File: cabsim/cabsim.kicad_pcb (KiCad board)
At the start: 2 copper layers, 87 x 30 mm, 45 parts, among them J1 NJ3FD-V, J3 Conn_01x01, J4 Conn_01x01, J5 NJ3FD-V, U3 Op_Amp_Dual, U4 Opamp_Quad

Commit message: update pcb
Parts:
- C4: value 1n -> 3.3n
- C7: value 2.2n -> 3.3n
- R19: value 390 -> 330
- R5, R9: value 3.9k -> 3.3k
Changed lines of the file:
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@@
 			)
 		)
-		(property "Value" "390"
+		(property "Value" "330"
 			(at 3.81 2.31 90)
 			(layer "F.Fab")
@@
 			)
 		)
-		(property "Value" "3.9k"
+		(property "Value" "3.3k"
 			(at 3.81 2.31 90)
 			(layer "F.Fab")
@@
 			)
 		)
-		(property "Value" "3.9k"
+		(property "Value" "3.3k"
 			(at 3.81 2.31 90)
 			(layer "F.Fab")
@@
 			)
 		)
-		(property "Value" "2.2n"
+		(property "Value" "3.3n"
 			(at 2.5 -2.31 90)
 			(layer "B.Fab")
@@
 			)
 		)
-		(property "Value" "1n"
+		(property "Value" "3.3n"
 			(at 2.5 -2.31 90)
 			(layer "B.Fab")

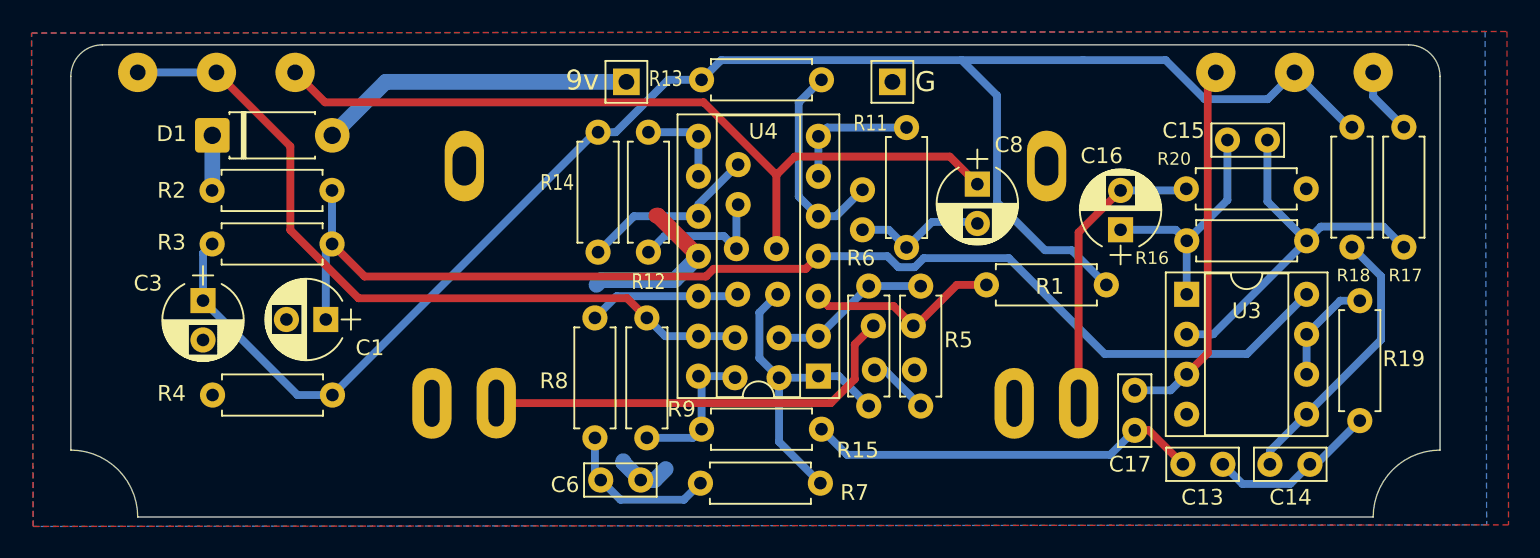
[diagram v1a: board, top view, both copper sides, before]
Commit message: update pcb and gitignore
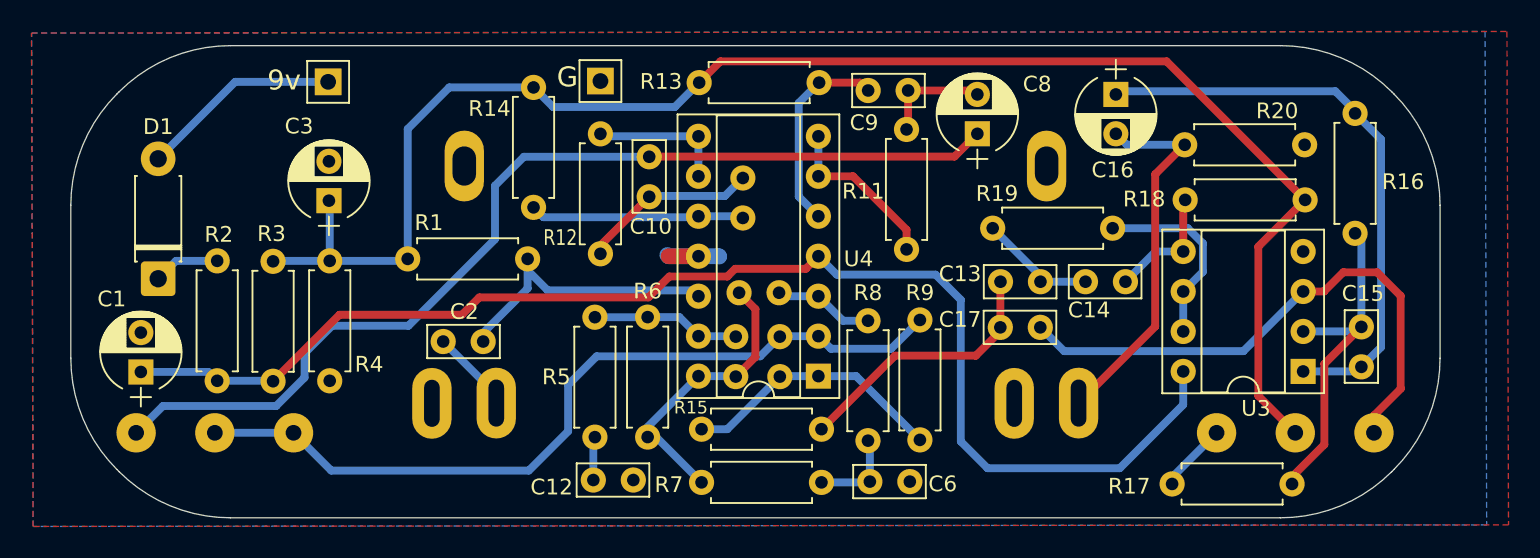
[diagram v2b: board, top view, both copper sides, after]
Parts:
- C10, C12, C2, C9: moved to F.Cu
- moved R1 29.2 mm to (111.5, 83.3), turned to 180 degrees
- moved C2 27.3 mm to (108.7, 88.6)
- moved R17 27.0 mm to (152.5, 97.7), turned to 0 degrees
- moved R19 26.3 mm to (141.1, 81.4), turned to 0 degrees
- moved R5 20.8 mm to (115.8, 94.7)
- moved C12 19.2 mm to (115.7, 97.4)
- moved J3 19.0 mm to (98.8, 72.1)
- moved J4 18.6 mm to (116.2, 72.0)
- moved C14 18.4 mm to (147.0, 84.8), turned to 0 degrees
- moved R8 17.4 mm to (133.2, 94.9)
- moved R9 17.4 mm to (136.4, 87.2)
- moved C6 17.1 mm to (133.3, 97.5)
- moved C13 16.4 mm to (141.6, 84.8)
- moved R6 14.2 mm to (119.2, 87.0)
- moved C15 13.3 mm to (164.5, 87.7), turned to -90 degrees
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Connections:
- C2 pad 1: Net-(U4A-+) -> Net-(U4D-+)
- C4 pad 2: Net-(U4A--) -> Net-(U4D--)
- C5 pad 1: Net-(U4D-+) -> Net-(U4A-+)
- C7 pad 2: Net-(U4D--) -> Net-(U4A--)
- R1 pad 1: Net-(U4A-+) -> Net-(U4D-+)
- R5 pad 2: Net-(U4A--) -> Net-(U4D--)
- R6 pad 1: Net-(U4A--) -> Net-(U4D--)
- R8 pad 2: Net-(U4D-+) -> Net-(U4A-+)
- R9 pad 1: Net-(U4D--) -> Net-(U4A--)
- RV1 pad 1: Net-(U4D--) -> Net-(U4A--)
- RV1 pad 2: Net-(U4D--) -> Net-(U4A--)
- U4 pad 1: Net-(C4-Pad1) -> Net-(C7-Pad1)
- U4 pad 14: Net-(C7-Pad1) -> Net-(C4-Pad1)
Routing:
- net Net-(U4A--): track 10.4 -> 52.1 mm
- net Net-(U4D--): track 48.0 -> 9.47 mm
- net Net-(C2-Pad2): track 27.3 -> 5.31 mm
- net Net-(C15-Pad2): track 15.4 -> 37.1 mm
- net Net-(C10-Pad1): track 51.9 -> 64.2 mm
- net Net-(U3A-+): track 23.7 -> 35.6 mm
- net Net-(U3B-+): track 17.5 -> 7.97 mm
- net GND: track 14.5 -> 5.25 mm
- net /vref: track 110.4 -> 101.2 mm
- net Net-(U4D-+): track 9.69 -> 18.7 mm
- net Net-(U3C-V+): track 76.3 -> 84.4 mm
- net Net-(C13-Pad1): track 25.2 -> 17.1 mm
- net Net-(C7-Pad1): track 9.52 -> 16.9 mm
- net Net-(D1-A): track 20.1 -> 12.8 mm
- net Net-(U4A-+): track 12.5 -> 6.39 mm
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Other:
- outline, holes or cut-outs redrawn
